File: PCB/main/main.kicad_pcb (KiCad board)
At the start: 2 copper layers, 100 x 100 mm, 46 parts, among them J1 Conn_01x33_Female, J2 Conn_01x33_Female, J3 Conn_01x33_Female, J4 Conn_01x33_Female, J5 USB_B_Micro, Q1 2N2222A, SW1 C13828, SW2 C13828, U1 TP4054, U2 MT3608L

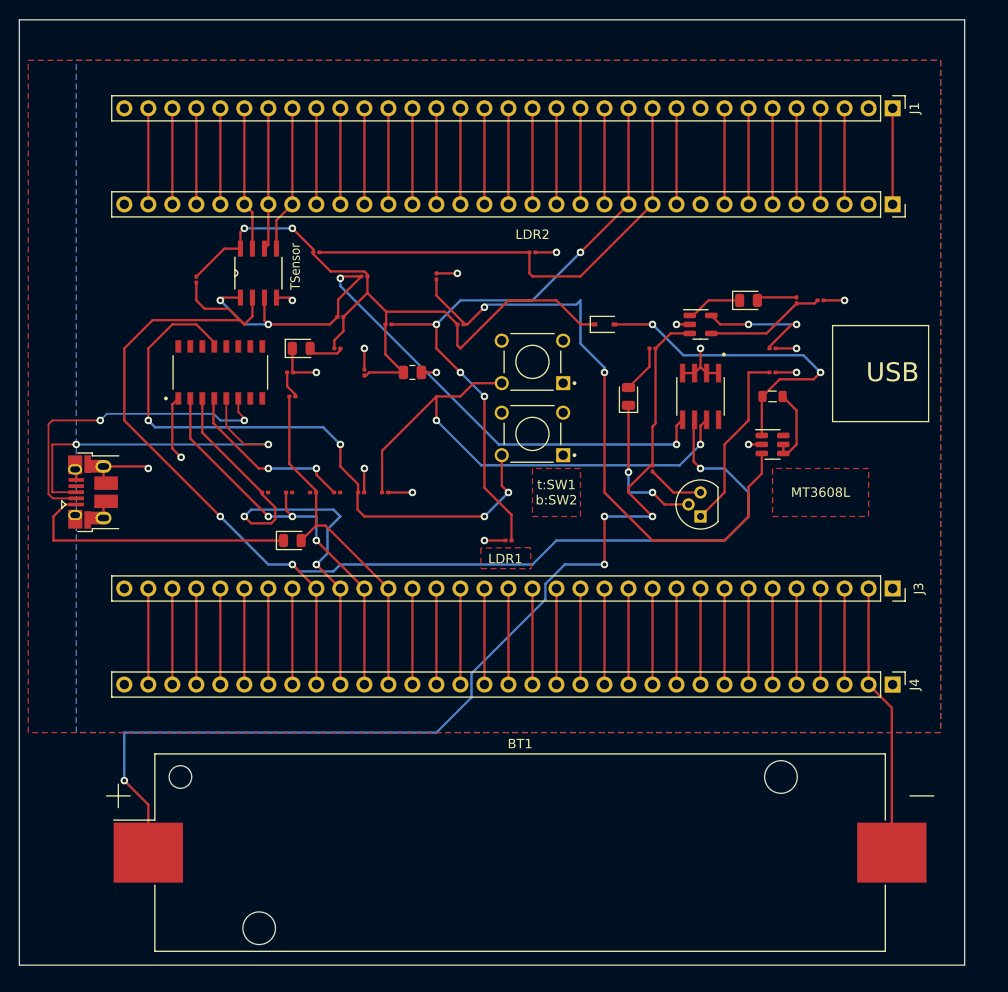
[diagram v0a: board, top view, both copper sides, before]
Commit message: updated PCB & Assembly file
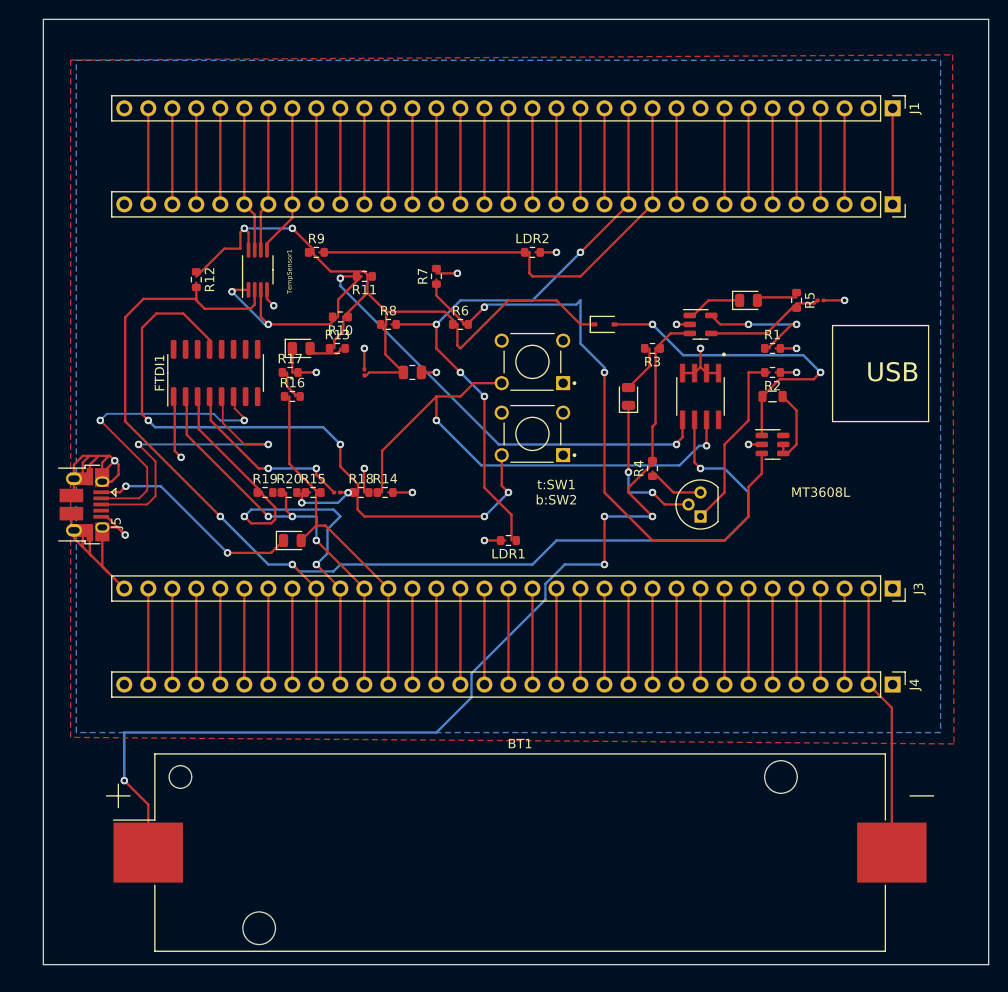
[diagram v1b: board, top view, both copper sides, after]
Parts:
- removed FTDI(UART)1: CH340C, CH340C:SOIC127P600X180-16N
- removed TSensor: LM75B, LM75BD:SOIC127P600X175-8N
- added FTDI1: CH340C, Package_SO:SOP-16_3.9x9.9mm_P1.27mm, F.Cu at (129.0, 78.8)
- added TempSensor1: LM75B, Package_SO:MSOP-8_3x3mm_P0.65mm, F.Cu at (133.5, 67.9)
- LDR1, LDR2, R1, R10, R11, R12, R13, R14, R15, R16, R17, R18, R19, R20, R5, R6, R7, R8, R9: footprint Resistor_SMD:R_0201_0603Metric -> Resistor_SMD:R_0603_1608Metric
- R2, R3, R4: value 100ohms -> 100; footprint Resistor_SMD:R_0201_0603Metric -> Resistor_SMD:R_0603_1608Metric
- moved J5 1.62 mm to (115.2, 92.7), turned to -90 degrees
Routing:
- net GND: track 83.8 -> 121.5 mm, vias 17 -> 18
- net +5V: track 0.00 -> 8.09 mm, vias 0 -> 2
- net /microcontroller_interfacing/USB Test Point: track 29.8 -> 23.0 mm, vias 0 -> 2
- net /PA8: track 135.9 -> 132.3 mm
- net USB D+: track 38.7 -> 35.1 mm
- net Net-(FTDI1-Pad13): track 67.5 -> 70.2 mm
- net /Power/Output: track 75.3 -> 77.8 mm
- net /PA9: track 50.4 -> 51.2 mm
- net /PA10: track 43.7 -> 44.5 mm
- net Net-(C4-Pad1): track 18.8 -> 19.6 mm
- net USB D-: track 34.6 -> 33.9 mm

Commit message: Updated PCB
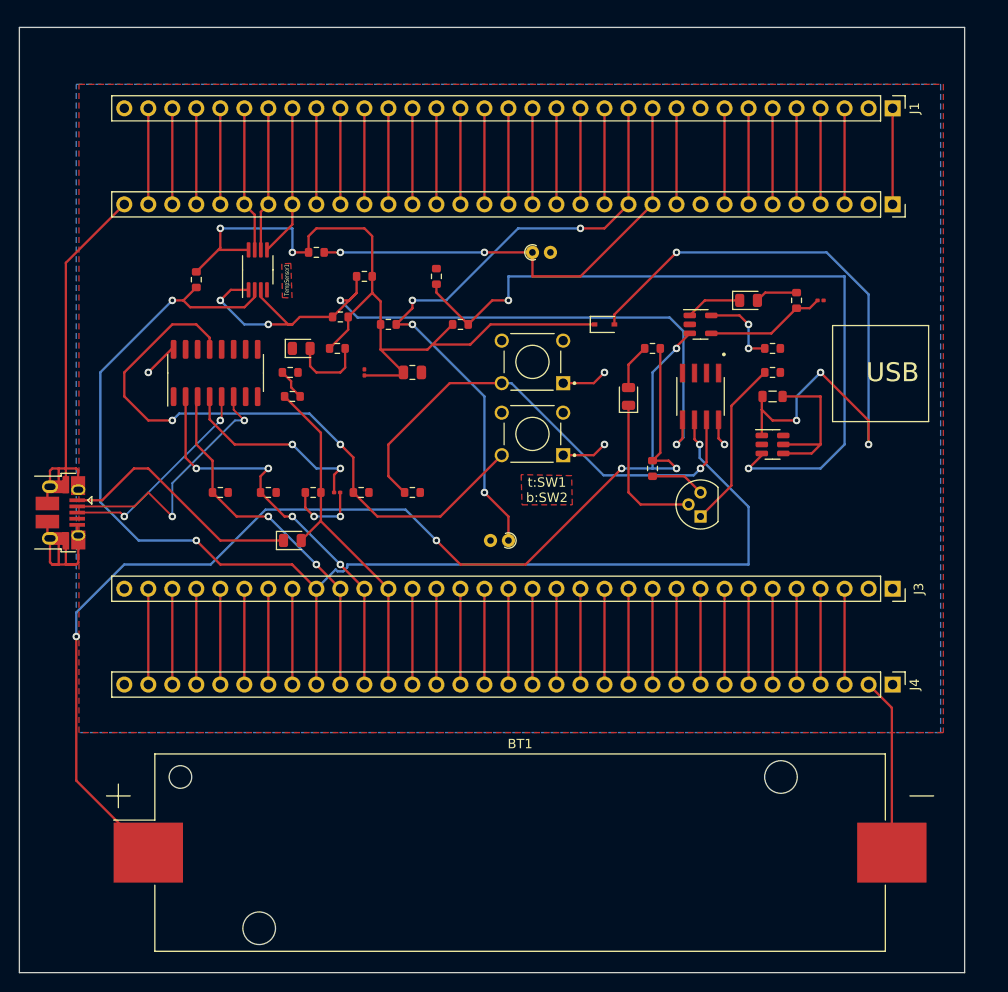
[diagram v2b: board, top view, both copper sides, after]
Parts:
- LDR1, LDR2: footprint Resistor_SMD:R_0603_1608Metric -> Resistor_THT:R_Axial_DIN0204_L3.6mm_D1.6mm_P1.90mm_Vertical
- moved R19 4.74 mm to (129.5, 91.4)
- moved R14 2.89 mm to (149.9, 91.4)
- moved J5 2.68 mm to (112.6, 93.6)
- moved R20 2.19 mm to (134.6, 91.4)
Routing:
- net GND: track 121.5 -> 79.5 mm, vias 18 -> 0
- net Net-(D3-Pad2): track 35.3 -> 72.5 mm, vias 2 -> 4
- net Net-(BT1-Pad1): track 108.9 -> 134.2 mm, vias 4 -> 5
- net +5V: track 8.09 -> 24.5 mm, vias 2 -> 6
- net Net-(R6-Pad2): track 66.6 -> 80.2 mm
- net USB D+: track 35.1 -> 22.1 mm
- net /PA9: track 51.2 -> 38.8 mm
- net /Sensing/I2CBUS: track 72.7 -> 82.2 mm
- net Net-(L1-Pad1): track 8.44 -> 17.4 mm
- net /Power/Output: track 77.8 -> 84.4 mm
- net /PA8: track 132.3 -> 138.2 mm
- net /microcontroller_interfacing/EEPROM MODE TP: track 56.7 -> 51.2 mm, vias 2 -> 1
- net USB D-: track 33.9 -> 28.6 mm
- net Net-(R1-Pad1): track 13.4 -> 8.59 mm
- net Net-(LED1-Pad2): track 3.75 -> 8.10 mm
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- added copper zone on B.Cu, net +5V
- added copper zone on F.Cu, net GND
- removed copper zone on F.Cu, net +5V
- removed copper zone on B.Cu, net GND
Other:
- board text removed: "MT3608L"
